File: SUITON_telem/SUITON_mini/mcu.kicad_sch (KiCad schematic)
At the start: 23 parts, among them J3 USB_C_Receptacle_USB2.0_16P, J4 Conn_01x06_Pin, U11 USBLC6-2P6, U5 STM32F405RGT6, X1 ABM3B-8.000MHZ-10-1UT

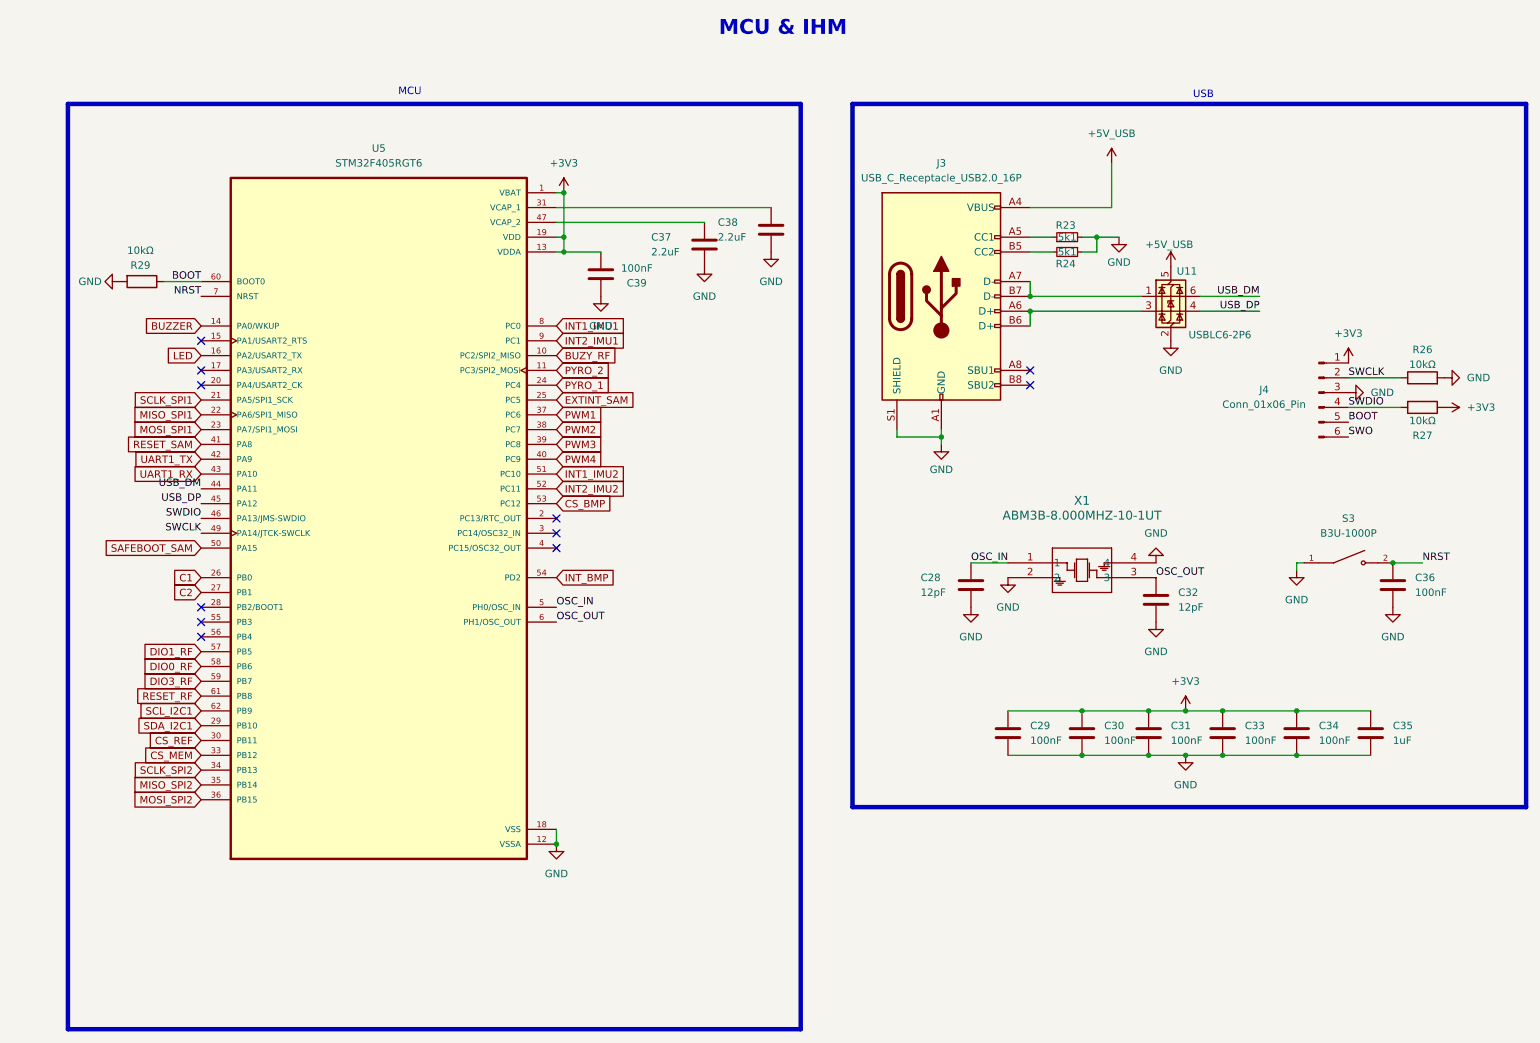
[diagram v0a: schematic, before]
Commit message: Shape
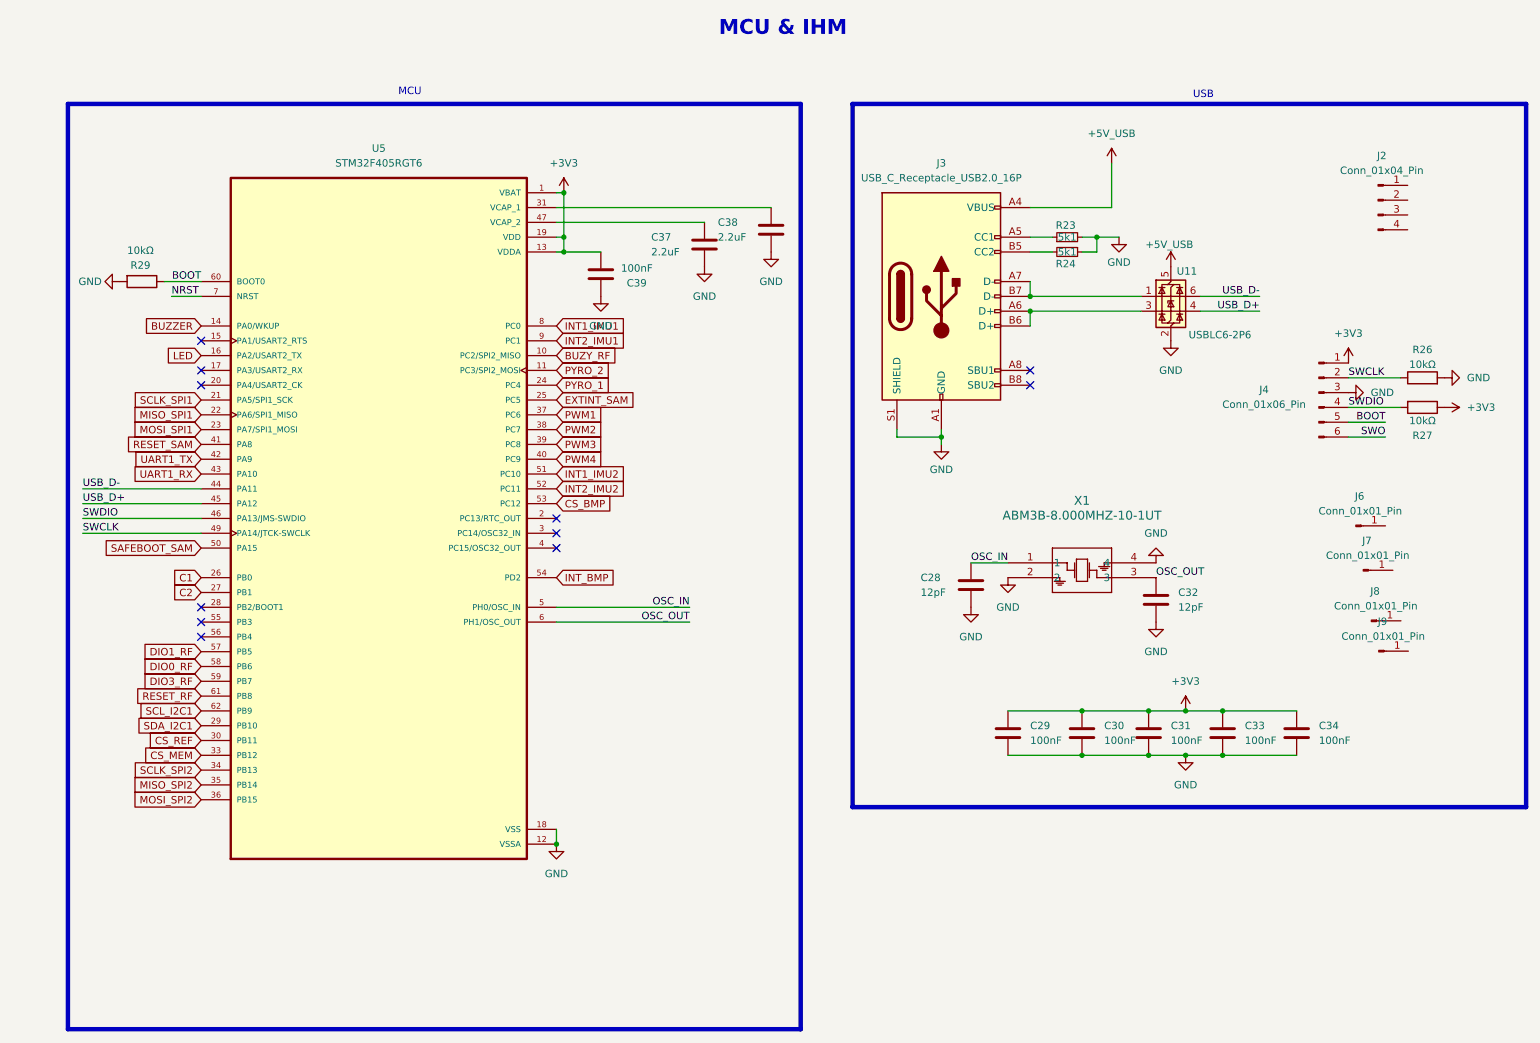
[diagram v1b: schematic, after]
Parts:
- removed C35: 1uF, Capacitor_SMD:C_0402_1005Metric, symbol Device:C
- removed C36: 100nF, Capacitor_SMD:C_0603_1608Metric, symbol Device:C
- removed S3: B3U-1000P, B3U-1000P:SW_B3U-1000P, symbol B3U-1000P:B3U-1000P
- added J2: Conn_01x04_Pin, Connector_JST:JST_SH_SM04B-SRSS-TB_1x04-1MP_P1.00mm_Horizontal, symbol Connector:Conn_01x04_Pin
- added J6, J7, J8, J9: Conn_01x01_Pin, Connector_Wire:SolderWirePad_1x01_SMD_1x2mm, symbol Connector:Conn_01x01_Pin
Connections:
- net USB_DM renamed USB_D-
- net USB_DP renamed USB_D+

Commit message: Suiton mini
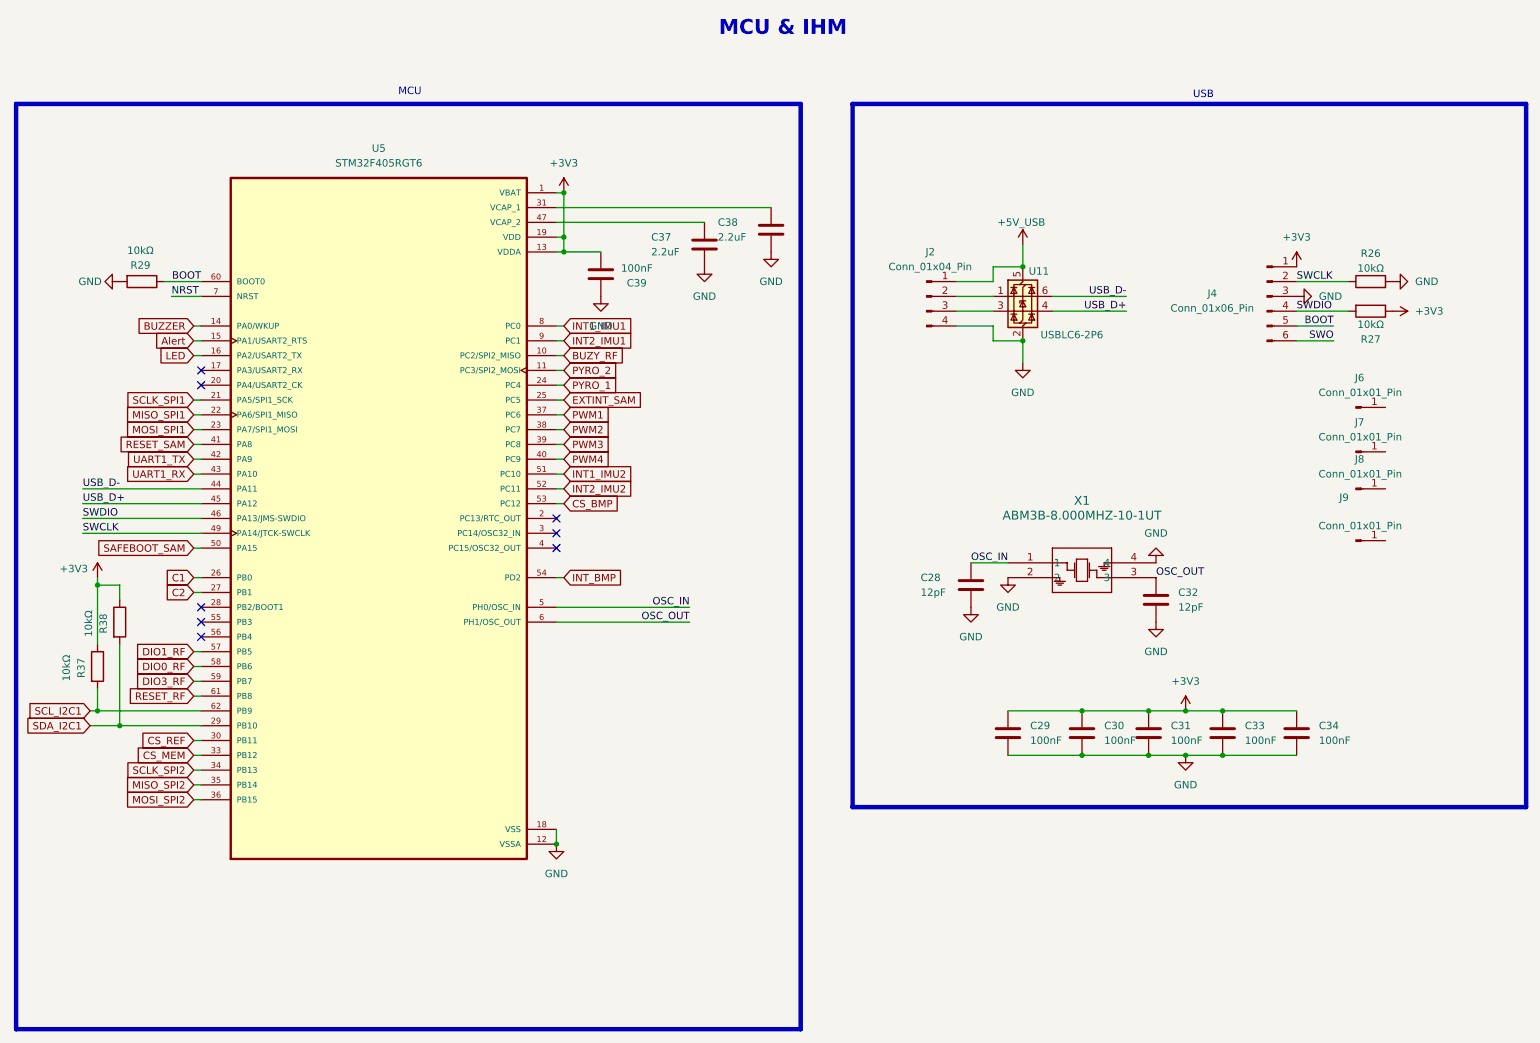
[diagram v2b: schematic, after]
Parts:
- removed J3: USB_C_Receptacle_USB2.0_16P, Connector_USB:USB_C_Receptacle_GCT_USB4105-xx-A_16P_TopMnt_Horizontal, symbol Connector:USB_C_Receptacle_USB2.0_16P
- removed R23, R24: 5k1, Resistor_SMD:R_0402_1005Metric, symbol Device:R_Small
- added R37, R38: 10kΩ, Resistor_SMD:R_0402_1005Metric, symbol Device:R
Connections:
- net +3V3: now also R37.1, R38.1
- net +5V_USB: now also J2.1 (Pin_1)
- net GND: now also J2.4 (Pin_4)
- net SCL_I2C1: now also R37.2
- net SDA_I2C1: now also R38.2
- net Alert: now reaches U5.15 (PA1/USART2_RTS)
- net at J2.2 (Pin_2): now also U11.1 (I/O1)
- net at J2.3 (Pin_3): now also U11.3 (I/O2)
- no-connect marks 11 -> 8
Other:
- moved on the sheet: J2, J4, J6, J7, J8, J9, R26, R27, U11
